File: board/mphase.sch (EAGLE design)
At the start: 31 parts, among them IC1 MAX232, IC2 PIC18F4455_40, X1 332-10, X2 332-10

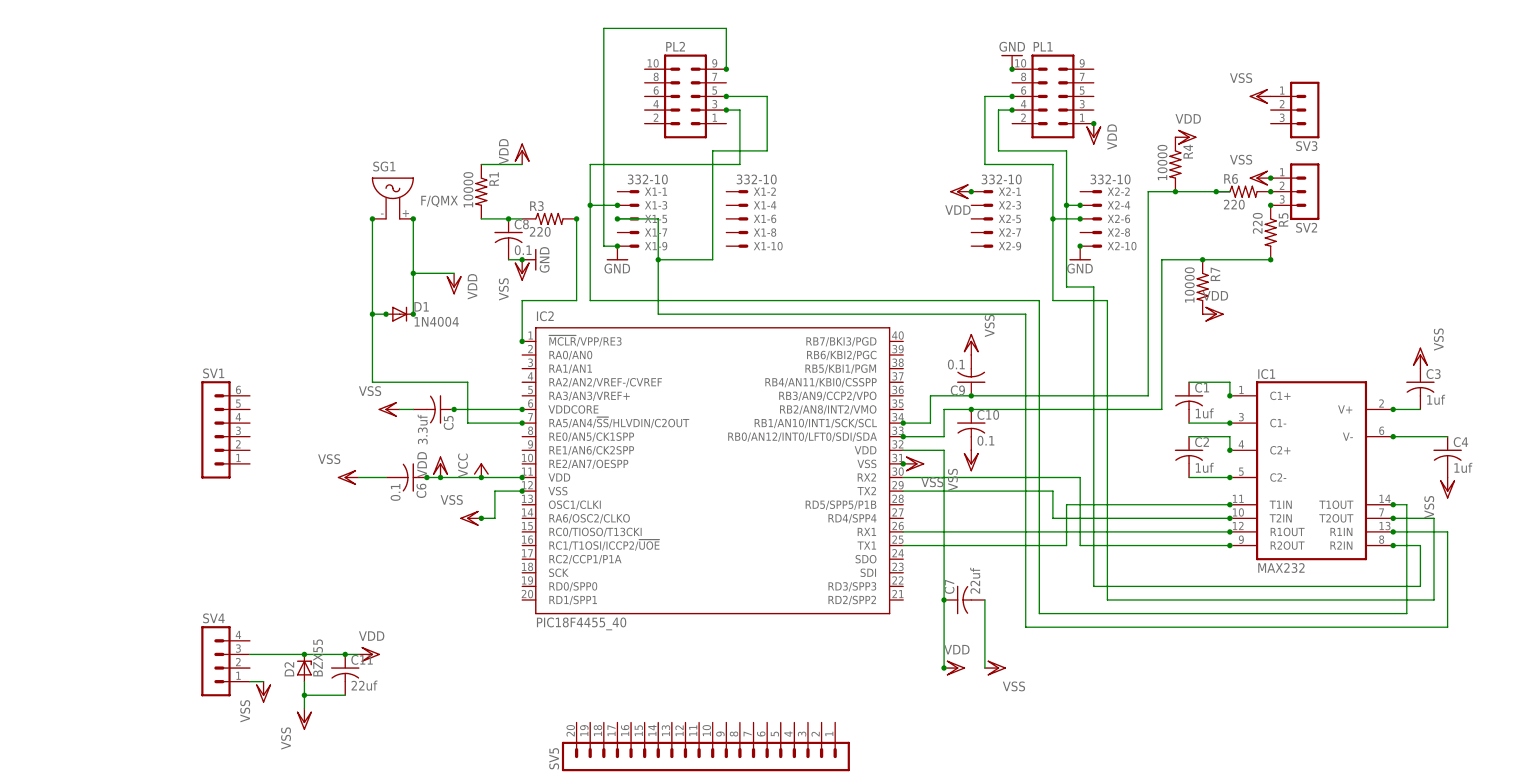
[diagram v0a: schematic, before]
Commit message: updates
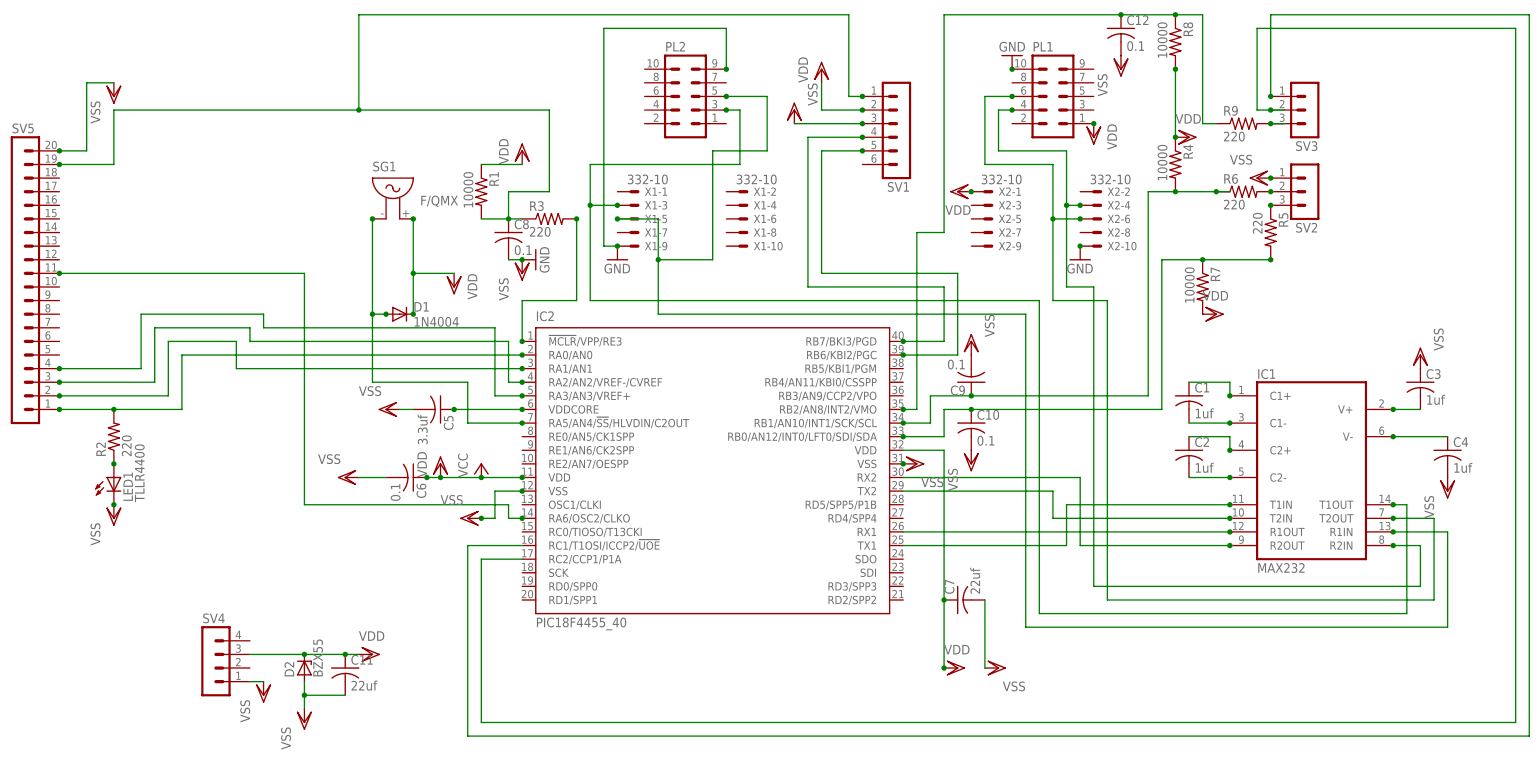
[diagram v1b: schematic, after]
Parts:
- added C12: 0.1, resistor:C-US025-024X044
- added LED1: TLLR4400, led:TLLR4400
- added R2, R9: 220, resistor:R-US_0204/2V
- added R8: 10000, resistor:R-US_0204/2V
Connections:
- new net N$15: IC2.RA0/AN0, R2.2, SV5.1
- new net N$18: LED1.A, R2.1
- new net N$23: IC2.RA1/AN1, SV5.2
- new net N$26: IC2.RA2/AN2/VREF-/CVREF, SV5.3
- new net N$27: IC2.RA3/AN3/VREF+, SV5.4
- new net N$28: C12.1, IC2.RB2/AN8/INT2/VMO, R8.1, R9.1
- new net N$29: IC2.RB7/BKI3/PGD, SV1.4
- new net N$30: IC2.RA6/OSC2/CLKO, SV5.11
- new net N$31: R9.2, SV3.3
- new net N$32: IC2.RB6/KBI2/PGC, SV1.5
- new net N$33: IC2.RC1/T1OSI/ICCP2/!UOE, SV3.1
- new net N$34: IC2.RC2/CCP1/P1A, SV3.2
- net N$8: now also SV1.1, SV5.19
- net VDD: now also R8.2, SV1.2
- net VSS: now also C12.2, LED1.C, SV1.3, SV5.20; no longer SV3.1
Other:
- moved on the sheet: SV1, SV5
